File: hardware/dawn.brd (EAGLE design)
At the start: 63.2 x 62.2 mm, 50 parts, among them IC1 LM393N, IC2 AT90S2313P, IC3 DS1307, Q1 IRFU9024N, Q2 4Mhz, Q3 32.768kHz, T1 BC457B, T2 BC557B

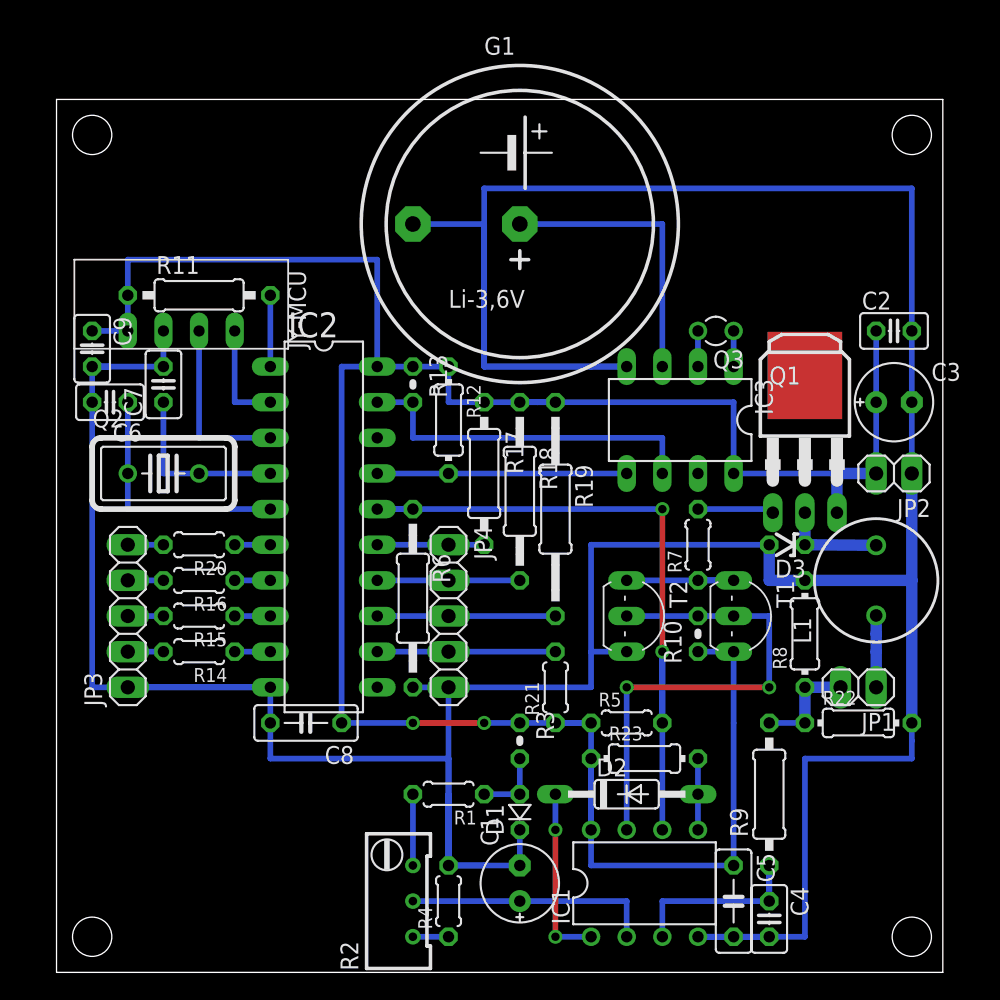
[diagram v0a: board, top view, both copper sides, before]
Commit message: Fixed schematic & board.
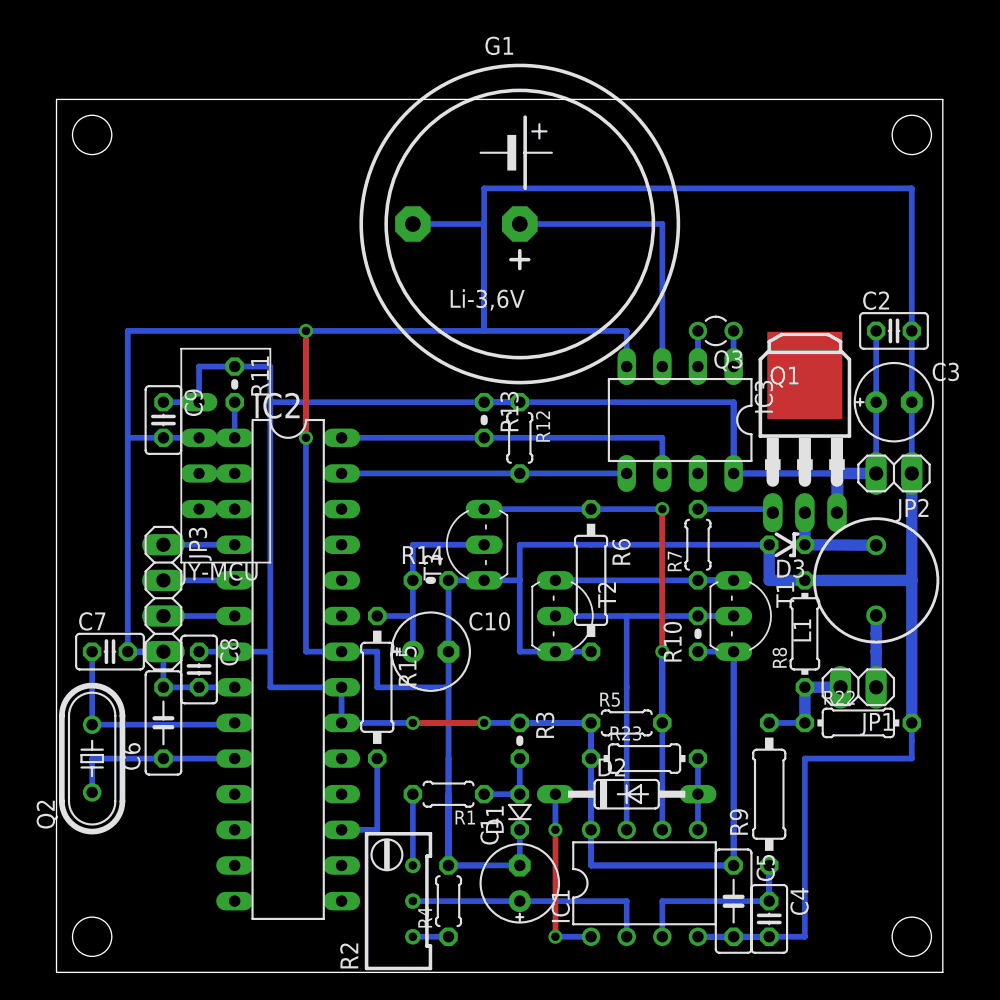
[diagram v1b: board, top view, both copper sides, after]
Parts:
- removed JP4: IN, pinhead:1X05
- removed R16, R20: 1.5k, rcl:0204/5
- removed R17: 10k, rcl:0207/10
- removed R18: 10k, rcl:0207/12
- removed R19: 10k, rcl:0207/15
- removed R21: 10k, rcl:0204/5
- added C10: 10uF, rcl:E2,5-6E
- added T3: BC457B, transistor:TO92-EBC
- C6: device rcl:C025-025X050 -> rcl:C050-025X075
- C8: device rcl:C050-025X075 -> rcl:C025-025X050
- IC2: value AT90S2313P -> ATMEGA168-20P; device atmel:DIL20 -> adafruit:DIL28-3
- JP3: value OUT -> (none); device pinhead:1X05 -> pinhead:1X04
- Q2: value 4Mhz -> 16MHz; device adafruit:HC18U-V -> crystal:HC49/S
- R11: device rcl:0207/10 -> rcl:0204V
- R12: device rcl:0204/7 -> rcl:0204/5
- R14: value 1.5k -> 10k; device rcl:0204/5 -> rcl:0204V
- R15: value 1.5k -> 15k; device rcl:0204/5 -> rcl:0207/10
- R6: device rcl:0207/12 -> rcl:0207/10
- moved C6 23.2 mm to (38.1, 33.0), turned to 90 degrees
- moved Q2 20.9 mm to (33.0, 30.5), turned to 90 degrees
- moved C7 19.4 mm to (34.3, 38.1), turned to 0 degrees
- moved R14 17.3 mm to (57.1, 43.2), turned to 0 degrees
- moved R15 13.7 mm to (53.3, 35.6), turned to 270 degrees
- moved R6 12.8 mm to (68.6, 43.2)
- moved IC2 10.5 mm to (47.0, 36.8)
- moved U$1 8.98 mm to (40.6, 52.1), turned to 0 degrees
- moved C8 8.52 mm to (40.6, 36.8), turned to 270 degrees
- moved C9 7.18 mm to (38.1, 54.6)
- moved R11 6.84 mm to (43.2, 57.1), turned to 270 degrees
- moved R13 5.68 mm to (61.0, 54.6)
- moved R12 5.24 mm to (63.5, 53.3)
- moved T2 5.08 mm to (67.3, 40.6)
- moved JP3 2.84 mm to (38.1, 41.9), turned to 270 degrees
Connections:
- removed net N$29: IC2.8, R15.1
- removed net N$31: IC2.15, JP4.1, R17.2
- removed net N$32: IC2.14, JP4.2, R18.2
- removed net N$33: IC2.13, JP4.3, R19.2
- removed net N$34: JP3.5, R20.2
- removed net N$35: IC2.6, R20.1
- removed net N$36: IC2.12, JP4.4, R21.2
- net +5V: now also IC2.21, IC2.7; no longer R17.1, R18.1, R19.1, R21.1
- net GND: now also C10.-, IC2.22, IC2.8, JP3.4, R14.2, T3.E; no longer IC2.10, JP3.1, JP4.5
- net N$12: now also IC2.3, U$1.RXD; no longer C7.1, IC2.4, Q2.2
- net N$18: now also IC2.10; no longer IC2.5
- net N$19: now also IC2.28; no longer IC2.19
- net N$21: now also IC2.27; no longer IC2.17
- net N$23: now also IC2.2; no longer IC2.3
- net N$24: now also IC2.4, JP3.1; no longer IC2.2, U$1.RXD
- net N$25: now also IC2.17, R15.2; no longer JP3.2, R14.2
- net N$26: now also C10.+, R14.1, R15.1, T3.B; no longer JP3.3, R15.2
- net N$27: now also IC2.5, JP3.2; no longer JP3.4, R16.2
- net N$28: now also IC2.6, JP3.3; no longer IC2.7, R16.1
- net N$30: now also C7.1, Q2.2; no longer R14.1
- net N$9: now also T3.C; no longer IC2.16
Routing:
- net +5V: track 184.9 -> 229.9 mm
- net GND: track 316.2 -> 336.6 mm, vias 0 -> 2
- net N$30: track 2.54 -> 15.5 mm
- net N$36: track 12.7 -> 0.00 mm
- net N$33: track 12.7 -> 0.00 mm
- net N$26: track 2.54 -> 15.2 mm
- net N$12: track 12.7 -> 2.54 mm
- net N$9: track 50.8 -> 40.6 mm
- net N$32: track 10.2 -> 0.00 mm
- net N$23: track 12.7 -> 2.54 mm
- net N$10: track 35.6 -> 27.9 mm, vias 2 -> 0
- net N$31: track 7.62 -> 0.00 mm
- net N$18: track 17.8 -> 12.6 mm
- net N$25: track 2.54 -> 7.62 mm
- net N$11: track 10.2 -> 15.2 mm
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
